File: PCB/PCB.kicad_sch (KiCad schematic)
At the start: 0 parts

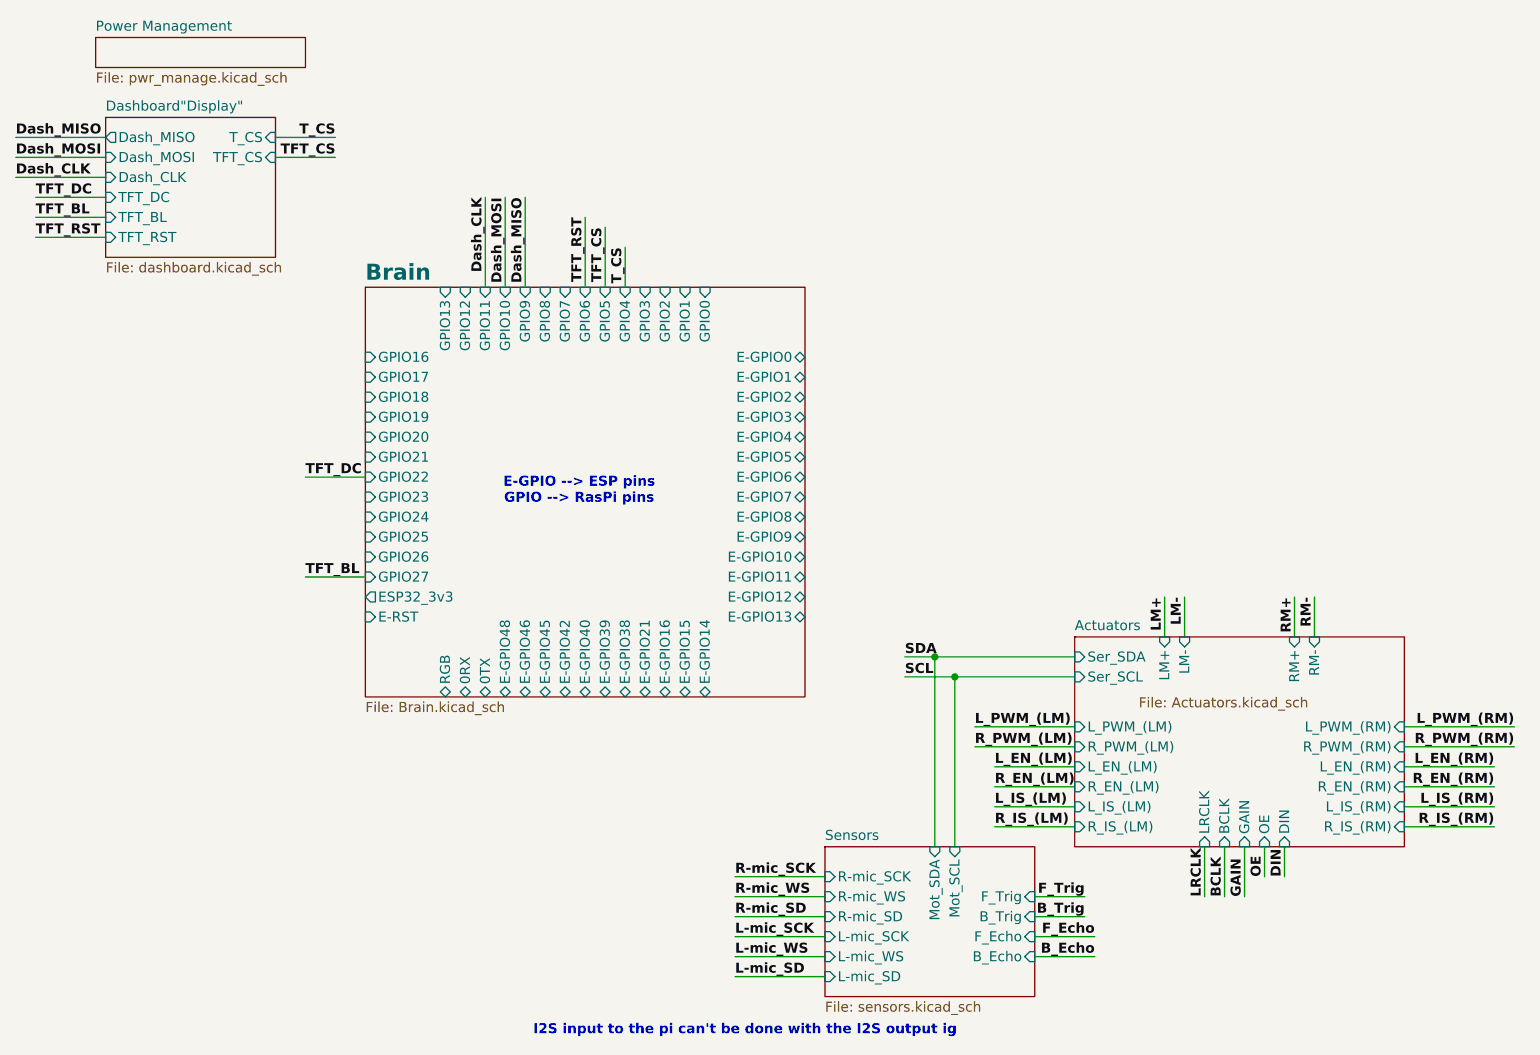
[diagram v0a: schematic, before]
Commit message: [PCB] Assigned all the footprints
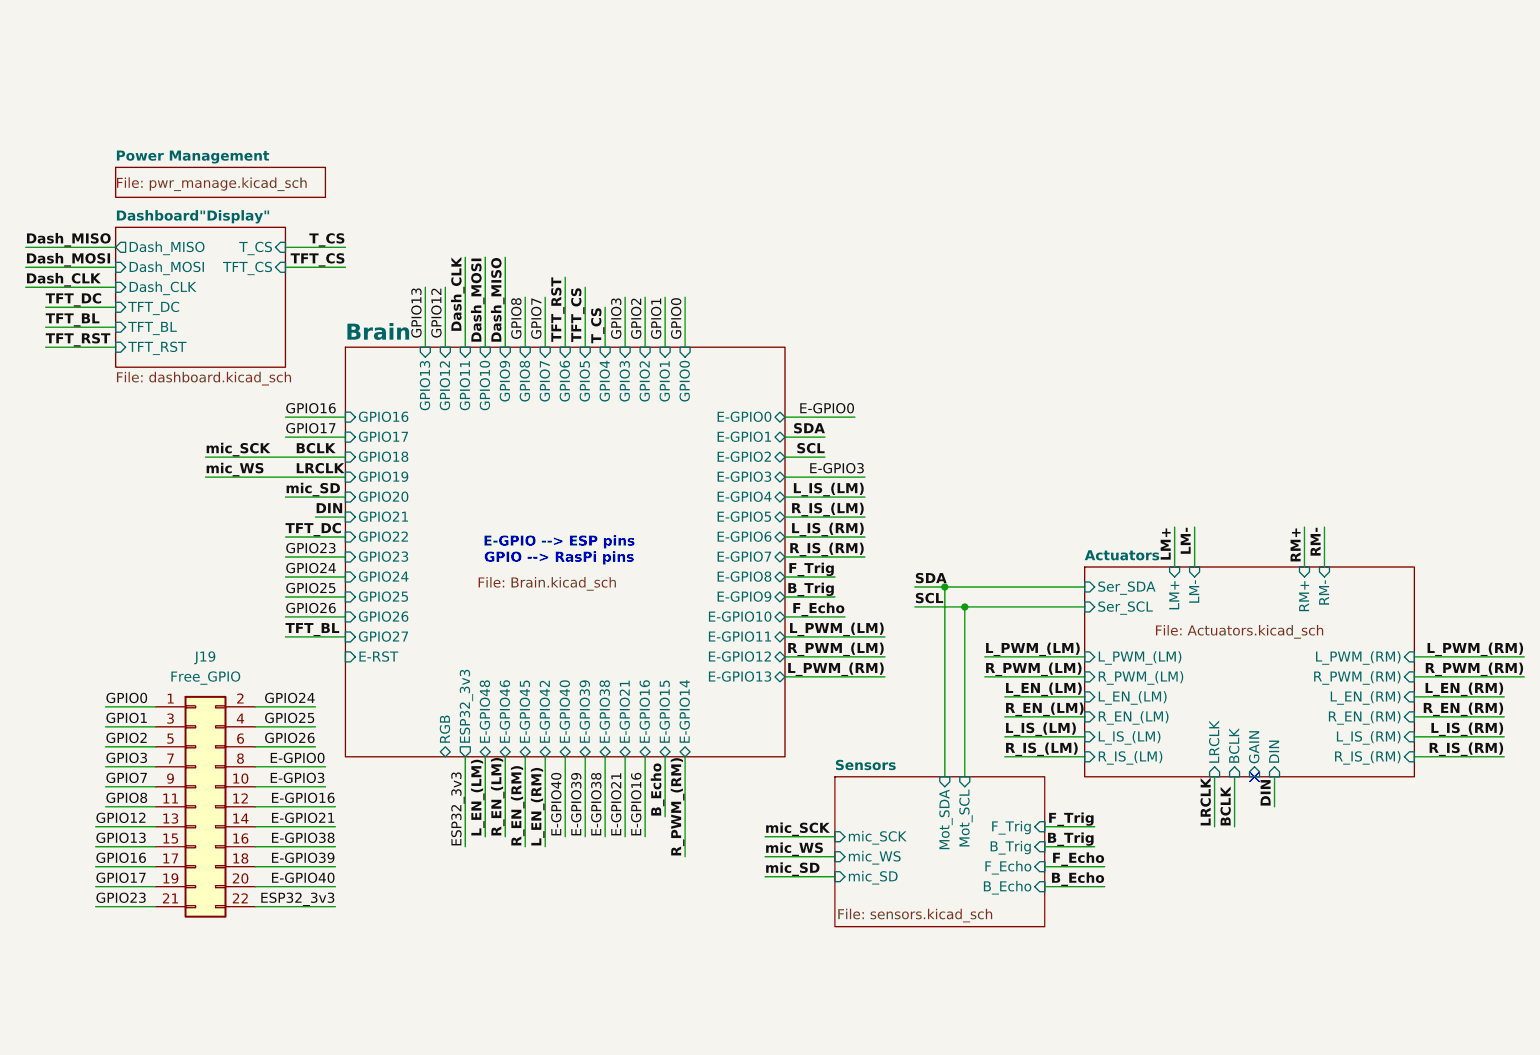
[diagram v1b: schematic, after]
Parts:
- added J19: Free_GPIO, Connector_PinHeader_2.54mm:PinHeader_2x11_P2.54mm_Vertical, symbol Connector_Generic:Conn_02x11_Odd_Even
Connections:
- new net E-GPIO0: J19.8 (Pin_8)
- new net E-GPIO16: J19.12 (Pin_12)
- new net E-GPIO21: J19.14 (Pin_14)
- new net E-GPIO3: J19.10 (Pin_10)
- new net E-GPIO38: J19.16 (Pin_16)
- new net E-GPIO39: J19.18 (Pin_18)
- new net E-GPIO40: J19.20 (Pin_20)
- new net ESP32_3v3: J19.22 (Pin_22)
- new net GPIO0: J19.1 (Pin_1)
- new net GPIO1: J19.3 (Pin_3)
- new net GPIO12: J19.13 (Pin_13)
- new net GPIO13: J19.15 (Pin_15)
- new net GPIO16: J19.17 (Pin_17)
- new net GPIO17: J19.19 (Pin_19)
- new net GPIO2: J19.5 (Pin_5)
- new net GPIO23: J19.21 (Pin_21)
- new net GPIO24: J19.2 (Pin_2)
- new net GPIO25: J19.4 (Pin_4)
- new net GPIO26: J19.6 (Pin_6)
- new net GPIO3: J19.7 (Pin_7)
- new net GPIO7: J19.9 (Pin_9)
- new net GPIO8: J19.11 (Pin_11)
- no-connect marks 0 -> 1
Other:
- sheet Actuators ports: added none; removed OE
- sheet Brain ports: added none; removed 0RX, 0TX
- sheet Sensors ports: added mic_SCK, mic_SD, mic_WS; removed L-mic_SCK, L-mic_SD, L-mic_WS, R-mic_SCK, R-mic_SD, R-mic_WS
- note removed: "I2S input to the pi can't be done with the I2S output ig"
